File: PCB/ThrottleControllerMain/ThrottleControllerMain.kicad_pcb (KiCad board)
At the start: 2 copper layers, 39 parts, among them J1 Conn_ARM_JTAG_SWD_10, J2 Conn_01x02, J4 Conn_01x04_Pin, J5 Screw_Terminal_01x02, J6 Screw_Terminal_01x02, P1 USB_C_Plug, U1 RP2040, U2 TLV493D, U3 NCP1117-3.3_SOT223, U5 W25Q32JVSS, Y1 12M

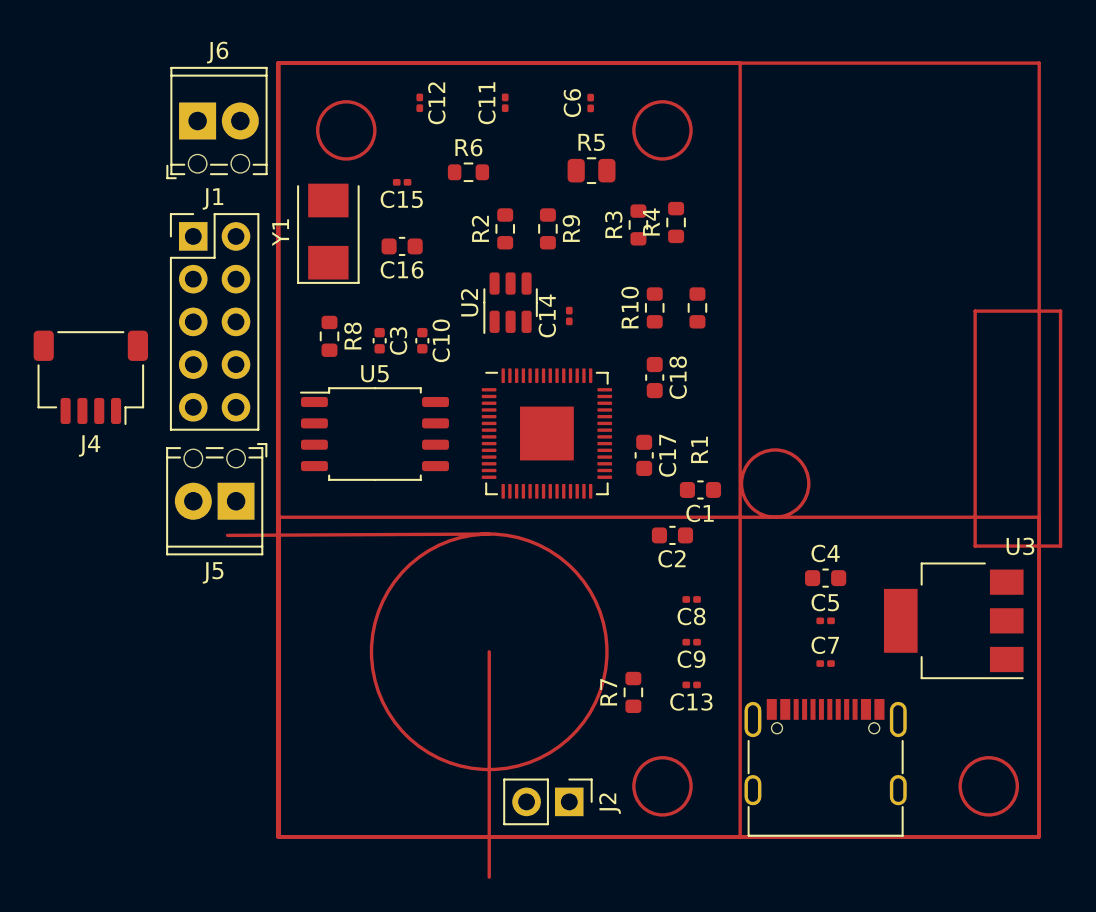
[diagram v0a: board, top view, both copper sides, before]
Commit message: PCB footprint layout is mostly complete.
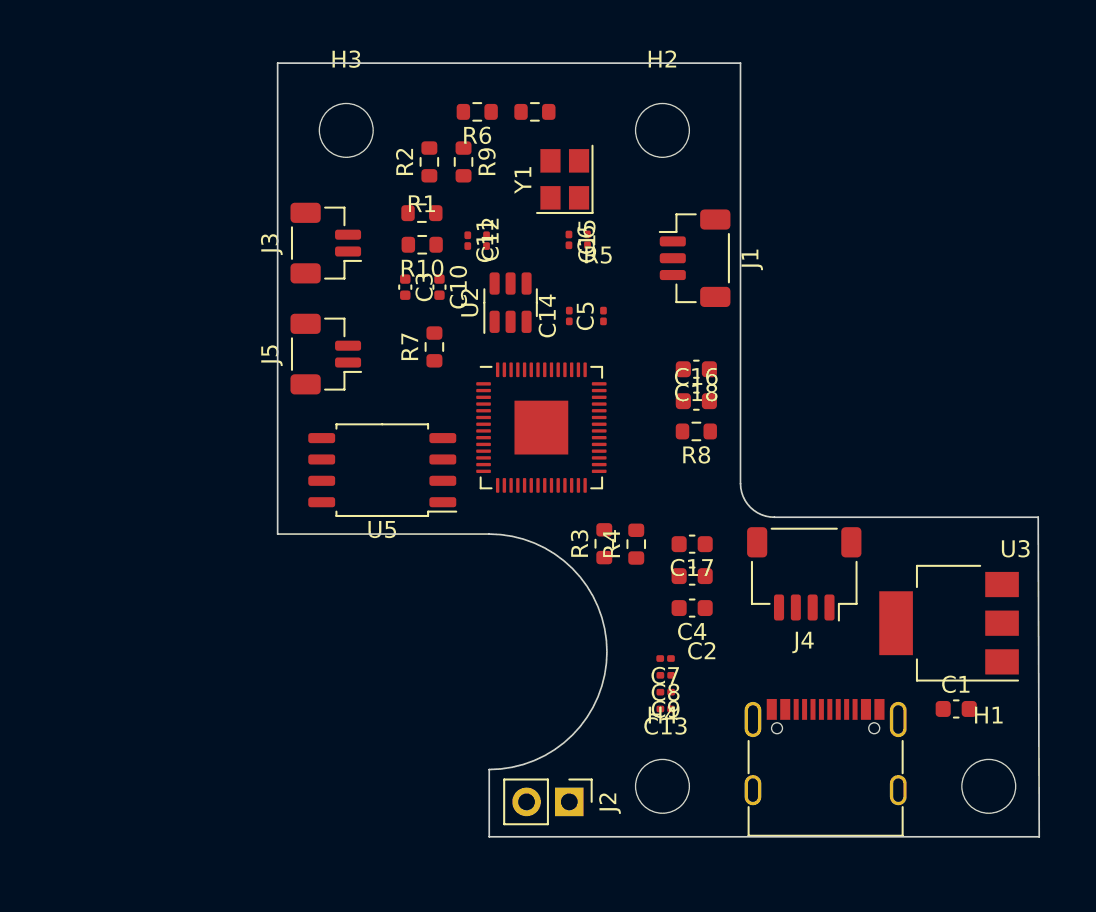
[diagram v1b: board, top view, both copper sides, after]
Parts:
- removed J6: Screw_Terminal_01x02, TerminalBlock_Phoenix:TerminalBlock_Phoenix_MPT-0,5-2-2.54_1x02_P2.54mm_Horizontal
- added H1: MountingHole, MountingHole:MountingHole_3.2mm_M3, F.Cu at (159.6, 108.9)
- added H2: MountingHole, MountingHole:MountingHole_3.2mm_M3, F.Cu at (140.2, 69.9)
- added H3: MountingHole, MountingHole:MountingHole_3.2mm_M3, F.Cu at (121.4, 69.9)
- added H4: MountingHole, MountingHole:MountingHole_3.2mm_M3, F.Cu at (140.2, 108.9)
- added J3: Conn_01x02_Socket, Connector_JST:JST_SH_BM02B-SRSS-TB_1x02-1MP_P1.00mm_Vertical, F.Cu at (120.1, 76.6)
- J1: value Conn_ARM_JTAG_SWD_10 -> Conn_01x03_Socket; footprint Connector_PinHeader_2.54mm:PinHeader_2x05_P2.54mm_Vertical -> Connector_JST:JST_SH_BM03B-SRSS-TB_1x03-1MP_P1.00mm_Vertical
- J5: value Screw_Terminal_01x02 -> Conn_01x02_Socket; footprint TerminalBlock_Phoenix:TerminalBlock_Phoenix_MPT-0,5-2-2.54_1x02_P2.54mm_Horizontal -> Connector_JST:JST_SH_BM02B-SRSS-TB_1x02-1MP_P1.00mm_Vertical
- R5: footprint Resistor_SMD:R_0805_2012Metric -> Resistor_SMD:R_0603_1608Metric
- Y1: footprint Crystal:Crystal_SMD_5032-2Pin_5.0x3.2mm -> Crystal:Crystal_SMD_3225-4Pin_3.2x2.5mm
- moved J4 44.0 mm to (148.6, 96.3)
- moved J1 29.9 mm to (142.1, 77.5), turned to -90 degrees
- moved R7 23.7 mm to (126.6, 82.8)
- moved R8 22.5 mm to (142.2, 87.8), turned to 180 degrees
- moved C5 22.4 mm to (136.7, 80.9), turned to 90 degrees
- moved C1 20.0 mm to (157.6, 104.3), turned to 0 degrees
- moved C16 19.8 mm to (142.2, 86.0), turned to 0 degrees
- moved R4 19.3 mm to (138.6, 94.5)
- moved R3 19.1 mm to (136.7, 94.5)
- moved R1 17.3 mm to (125.9, 74.8), turned to 0 degrees
- moved Y1 14.4 mm to (134.3, 72.8)
- moved R10 14.3 mm to (125.9, 76.7), turned to 180 degrees
- moved C15 11.5 mm to (135.7, 76.4), turned to 90 degrees
- moved J5 10.2 mm to (120.1, 83.2), turned to 90 degrees
- moved C7 9.52 mm to (140.3, 101.3), turned to 180 degrees
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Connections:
- J1 pad 1: +3.3V -> GND
- J1 pad 3: GND -> Net-(J1-Pin_3)
- R10 pad 2: Net-(J6-Pin_1) -> Net-(J5-Pin_1)
- R5 pad 2: Net-(J1-~{RESET}) -> Net-(U1-RUN)
- R9 pad 2: Net-(J5-Pin_1) -> Net-(J3-Pin_1)
- U1 pad 24: Net-(J1-SWDCLK/TCK) -> Net-(J1-Pin_3)
- U1 pad 26: Net-(J1-~{RESET}) -> Net-(U1-RUN)
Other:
- board outline added: 45.3 x 46 mm
